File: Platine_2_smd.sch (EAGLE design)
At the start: 19 parts, among them X2 DTF13-12PA

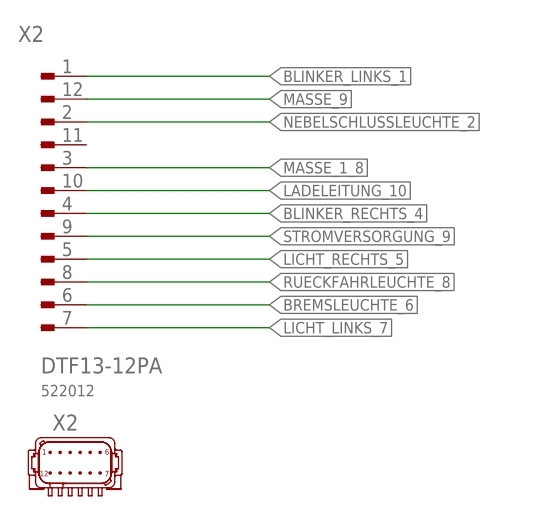
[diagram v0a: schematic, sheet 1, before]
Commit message: Diode added !
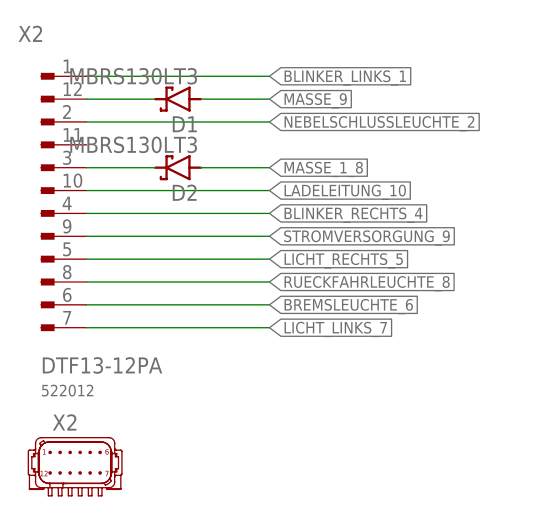
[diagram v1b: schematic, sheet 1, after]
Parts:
- added D1, D2: MBRS130LT3, diode:MBRS130LT3
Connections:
- new net N$10: D1.C, X2G$1.12
- new net N$11: D2.C, X2G$1.3
- net MASSE_1_8: now also D2.A; no longer X2G$1.3
- net MASSE_9: now also D1.A; no longer X2G$1.12
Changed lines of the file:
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@@
 <part name="FRAME1" library="frames" library_urn="urn:adsk.eagle:library:229" deviceset="A4P-LOC" device=""/>
 <part name="FRAME2" library="frames" library_urn="urn:adsk.eagle:library:229" deviceset="A4P-LOC" device=""/>
+<part name="D1" library="diode" library_urn="urn:adsk.eagle:library:210" deviceset="MBRS130LT3" device="" package3d_urn="urn:adsk.eagle:package:43404/2"/>
+<part name="D2" library="diode" library_urn="urn:adsk.eagle:library:210" deviceset="MBRS130LT3" device="" package3d_urn="urn:adsk.eagle:package:43404/2"/>
 </parts>
 <sheets>
@@
 <attribute name="LAST_DATE_TIME" x="140.97" y="10.16" size="2.286" layer="94"/>
 <attribute name="SHEET" x="154.305" y="5.08" size="2.54" layer="94"/>
+</instance>
+<instance part="D1" gate="G$1" x="33.02" y="63.5" smashed="yes" rot="R180">
+<attribute name="NAME" x="35.306" y="61.595" size="1.778" layer="95" rot="R180"/>
+<attribute name="VALUE" x="35.306" y="66.929" size="1.778" layer="96" rot="R180"/>
+</instance>
+<instance part="D2" gate="G$1" x="33.02" y="55.88" smashed="yes" rot="R180">
+<attribute name="NAME" x="35.306" y="53.975" size="1.778" layer="95" rot="R180"/>
+<attribute name="VALUE" x="35.306" y="59.309" size="1.778" layer="96" rot="R180"/>
 </instance>
 </instances>
@@
 <net name="MASSE_1_8" class="0">
 <segment>
-<pinref part="X2" gate="G$1" pin="3"/>
-<wire x1="22.86" y1="55.88" x2="43.18" y2="55.88" width="0.1524" layer="91"/>
 <label x="43.18" y="55.88" size="1.27" layer="95" xref="yes"/>
+<wire x1="35.56" y1="55.88" x2="43.18" y2="55.88" width="0.1524" layer="91"/>
+<pinref part="D2" gate="G$1" pin="A"/>
 </segment>
 </net>
 <net name="MASSE_9" class="0">
 <segment>
-<pinref part="X2" gate="G$1" pin="12"/>
-<wire x1="22.86" y1="63.5" x2="43.18" y2="63.5" width="0.1524" layer="91"/>
 <label x="43.18" y="63.5" size="1.27" layer="95" xref="yes"/>
+<wire x1="35.56" y1="63.5" x2="43.18" y2="63.5" width="0.1524" layer="91"/>
+<pinref part="D1" gate="G$1" pin="A"/>
 </segment>
 </net>
+<net name="N$10" class="0">
+<segment>
+<pinref part="X2" gate="G$1" pin="12"/>
+<wire x1="22.86" y1="63.5" x2="30.48" y2="63.5" width="0.1524" layer="91"/>
+<pinref part="D1" gate="G$1" pin="C"/>
+</segment>
+</net>
+<net name="N$11" class="0">
+<segment>
+<pinref part="X2" gate="G$1" pin="3"/>
+<wire x1="22.86" y1="55.88" x2="30.48" y2="55.88" width="0.1524" layer="91"/>
+<pinref part="D2" gate="G$1" pin="C"/>
+</segment>
+</net>
